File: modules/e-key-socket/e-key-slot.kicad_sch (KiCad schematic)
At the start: 0 parts

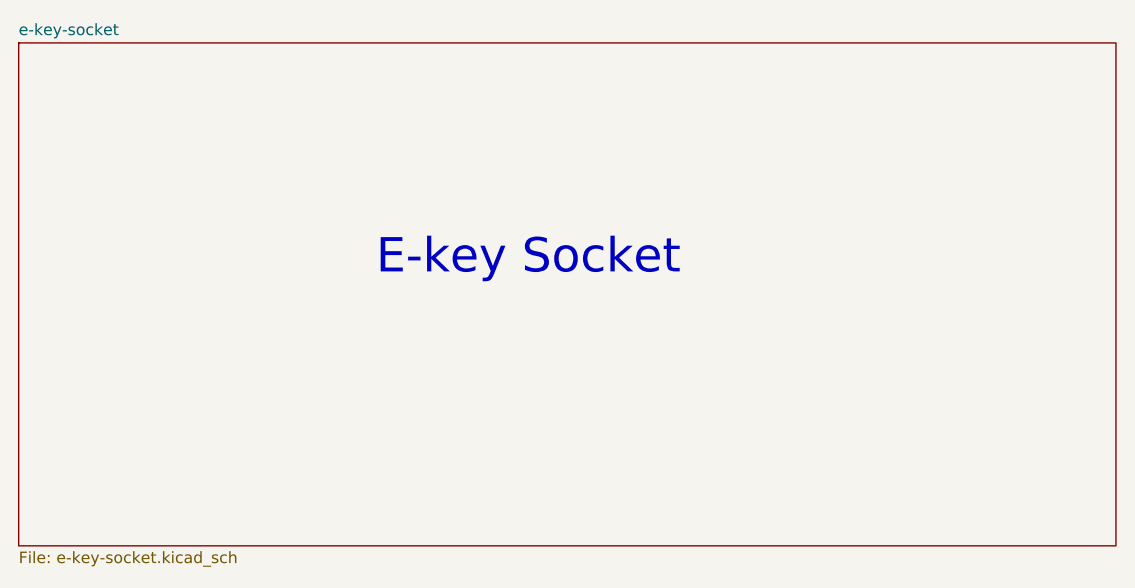
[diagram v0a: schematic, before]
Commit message: fix: text formatting and modify gitignore
Signed-off-by: Rodney Osodo <socials@rodneyosodo.com>
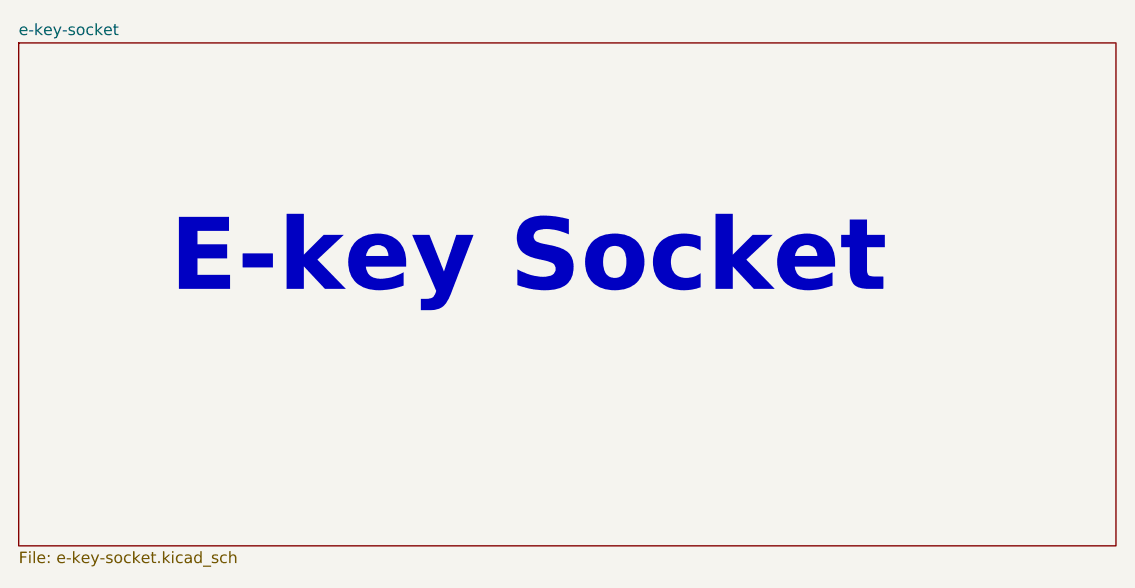
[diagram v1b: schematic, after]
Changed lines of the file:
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@@
 		(effects
 			(font
-				(size 3.81 3.81)
+				(size 8 8)
+				(thickness 1.6)
+				(bold yes)
 			)
 		)
